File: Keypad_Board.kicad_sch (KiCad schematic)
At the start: 44 parts, among them IC1 STM32L010K4T6, IC2 TMUX136RSER, J1 Data_Conn_Header, J2 Pin_Header, J3 Data_Conn_Socket, J4 SEL Jumper, J5 SW_Header, J6 BOOT Jumper

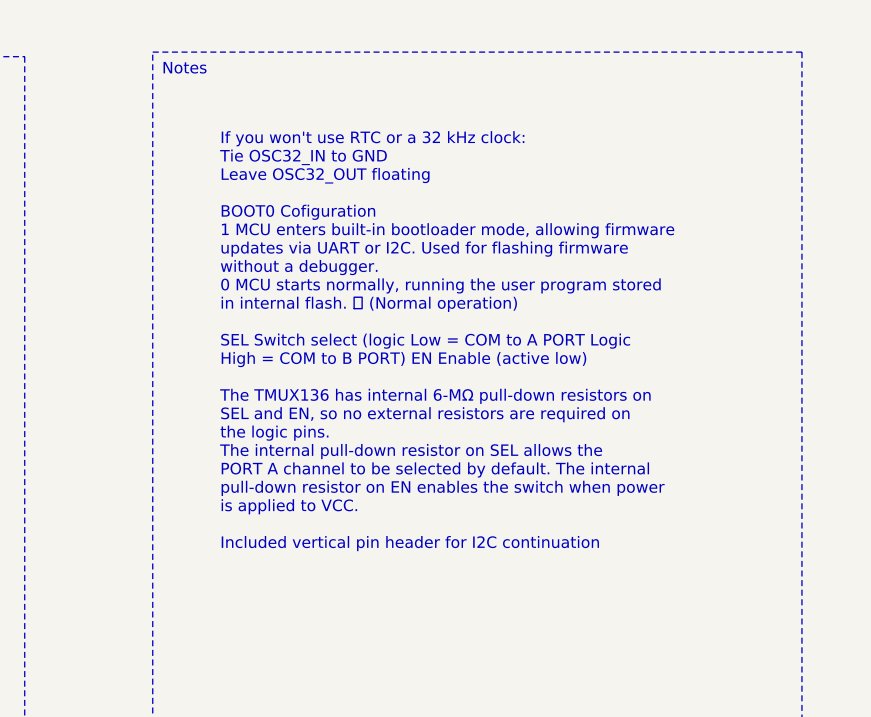
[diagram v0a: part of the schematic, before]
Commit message: Update
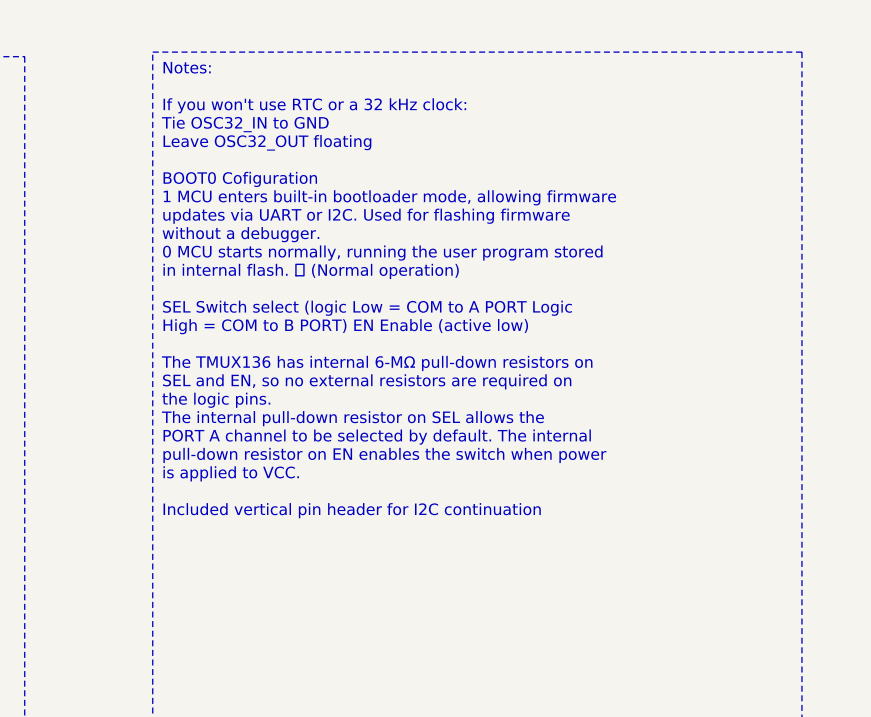
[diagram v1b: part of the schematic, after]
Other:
- note removed: "If you won't use RTC or a 32 kHz clock: Tie OSC32_IN to GND Leave OSC32_OUT floating BOOT0 Cofiguration 1 MCU enters built-in bootloader mode, allowing firmware updates via UART or I2C. Used for flashing firmware without a debugger. 0 MCU starts normally, running the user program stored in internal flash. ✅ (Normal operation) SEL Switch select (logic Low = COM to A PORT Logic High = COM to B PORT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"
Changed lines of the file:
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@@
 		)
 	)
-	(text_box "Notes"
+	(text_box "Notes:\n\nIf you won't use RTC or a 32 kHz clock:\nTie OSC32_IN to GND\nLeave OSC32_OUT floating\n\nBOOT0 Cofiguration\n1 MCU enters built-in bootloader mode, allowing firmware \nupdates via UART or I2C. Used for flashing firmware \nwithout a debugger.\n0 MCU starts normally, running the user program stored \nin internal flash. ✅ (Normal operation)\n\nSEL Switch select (logic Low = COM to A PORT Logic \nHigh = COM to B PORT) EN Enable (active low)\n\nThe TMUX136 has internal 6-MΩ pull-down resistors on \nSEL and EN, so no external resistors are required on \nthe logic pins. \nThe internal pull-down resistor on SEL allows the \nPORT A channel to be selected by default. The internal \npull-down resistor on EN enables the switch when power \nis applied to VCC.\n\nIncluded vertical pin header for I2C continuation"
 		(exclude_from_sim no)
 		(at 320.929 26.162 0)
@@
 		)
 	)
-	(text "If you won't use RTC or a 32 kHz clock:\nTie OSC32_IN to GND\nLeave OSC32_OUT floating\n\nBOOT0 Cofiguration\n1 MCU enters built-in bootloader mode, allowing firmware \nupdates via UART or I2C. Used for flashing firmware \nwithout a debugger.\n0 MCU starts normally, running the user program stored \nin internal flash. ✅ (Normal operation)\n\nSEL Switch select (logic Low = COM to A PORT Logic \nHigh = COM to B PORT) EN Enable (active low)\n\nThe TMUX136 has internal 6-MΩ pull-down resistors on \nSEL and EN, so no external resistors are required on \nthe logic pins. \nThe internal pull-down resistor on SEL allows the \nPORT A channel to be selected by default. The internal \npull-down resistor on EN enables the switch when power \nis applied to VCC.\n\nIncluded vertical pin header for I2C continuation"
-		(exclude_from_sim no)
-		(at 328.422 58.42 0)
-		(effects
-			(font
-				(size 1.27 1.27)
-			)
-			(justify left)
-		)
-	)
